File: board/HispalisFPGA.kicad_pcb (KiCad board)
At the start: 4 copper layers, 91.3 x 79.9 mm, 129 parts, among them J1 HC-TYPE-C-16P-01A, Q1 DMG1012T, Q2 DMG1012T, Q3 DMG1012T, Q4 DMG1012T, SW1 SW_DIP_x08, U1 93LC46B, U2 FT2232HQ, Y1 12MHz

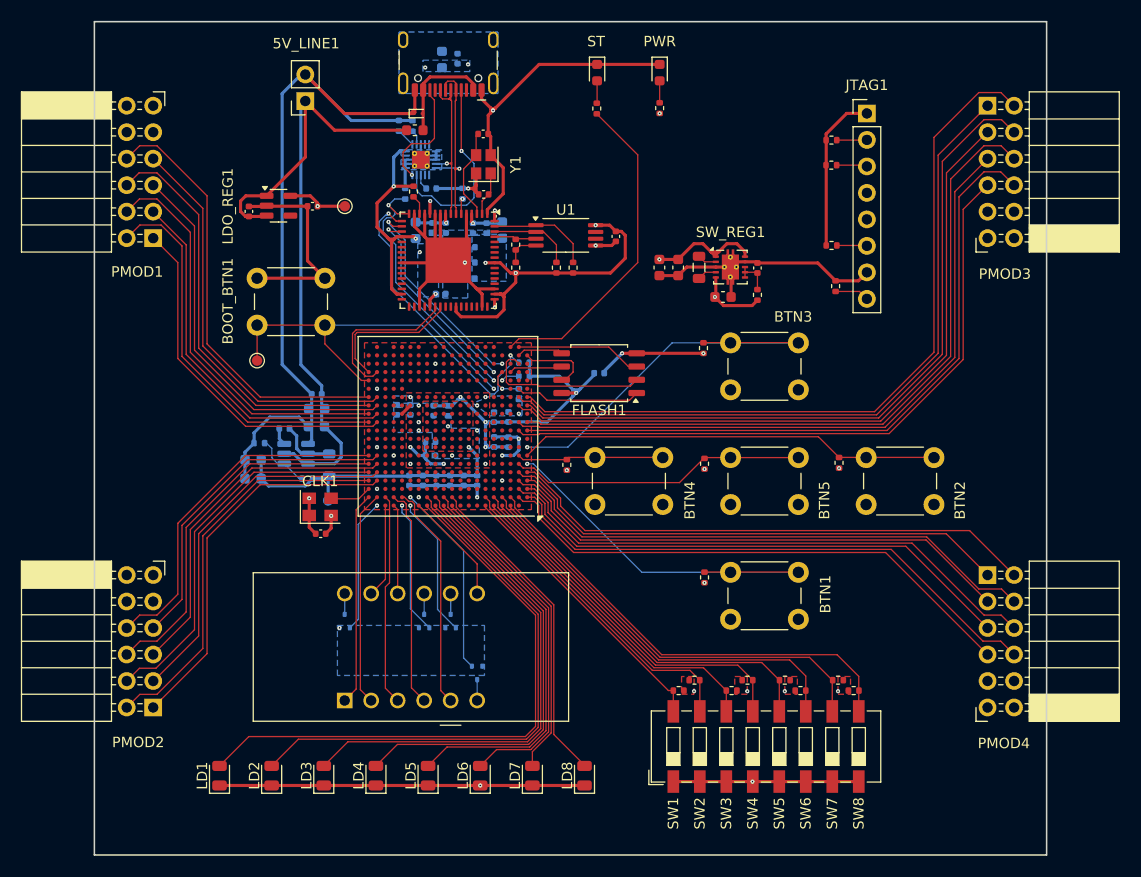
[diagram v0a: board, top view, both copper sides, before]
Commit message: No warnings
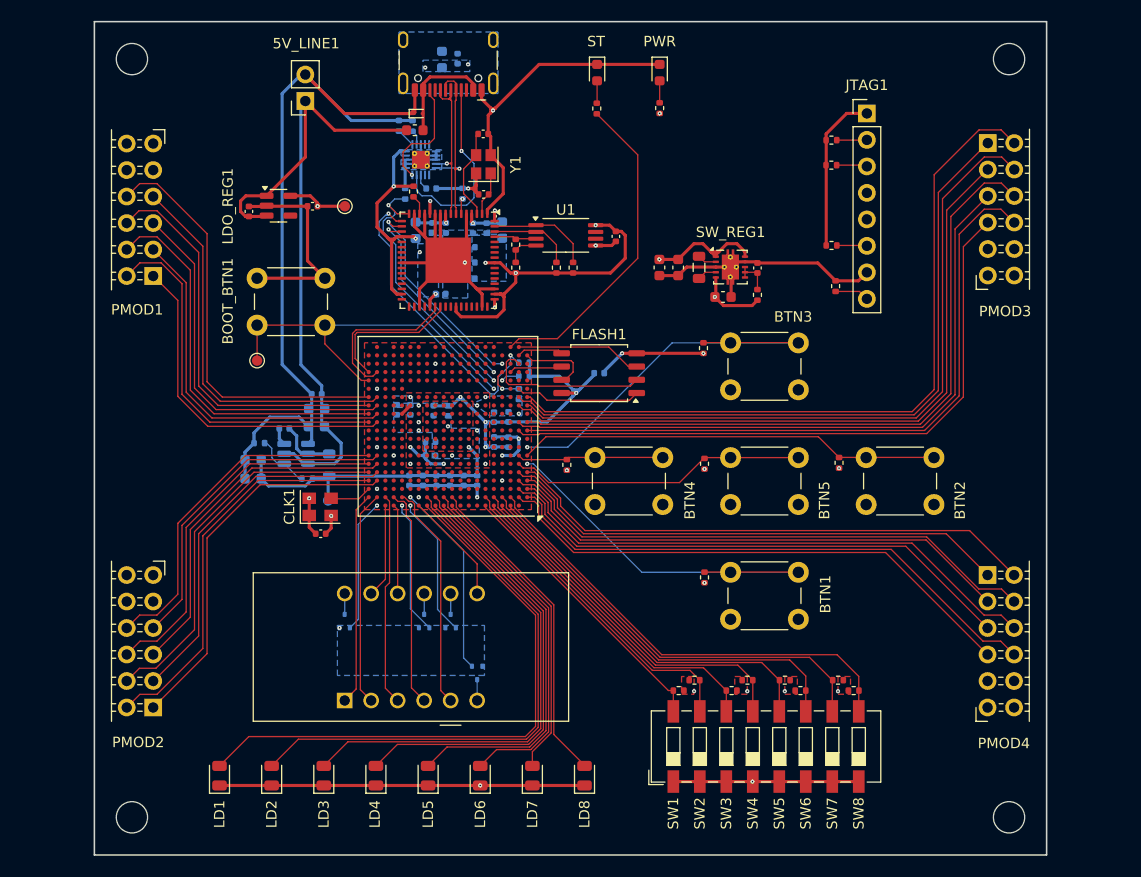
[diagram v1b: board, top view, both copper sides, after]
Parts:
- added MH01: MountingHole_3mm, MountingHole:MountingHole_3mm, F.Cu at (65.9, 107.0)
- added MH02: MountingHole_3mm, MountingHole:MountingHole_3mm, F.Cu at (150.0, 107.0)
- added MH03: MountingHole_3mm, MountingHole:MountingHole_3mm, F.Cu at (65.9, 179.7)
- added MH04: MountingHole_3mm, MountingHole:MountingHole_3mm, F.Cu at (150.0, 179.7)
- moved PMOD1 3.63 mm to (67.9, 115.1)
- moved PMOD3 3.58 mm to (148.0, 127.8)
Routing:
- net PMOD1_9: track 40.4 -> 38.9 mm
- net PMOD1_7: track 37.8 -> 36.3 mm
- net PMOD1_8: track 39.0 -> 37.5 mm
- net PMOD1_4: track 39.0 -> 37.5 mm
- net PMOD1_3: track 37.5 -> 36.0 mm
- net PMOD1_2: track 36.0 -> 34.5 mm
- net PMOD1_1: track 34.5 -> 33.0 mm
- net PMOD1_10: track 42.0 -> 40.5 mm
- net PMOD3_8: track 70.4 -> 68.9 mm
- net PMOD3_7: track 72.5 -> 71.1 mm
- net PMOD3_9: track 68.3 -> 66.8 mm
- net PMOD3_4: track 63.4 -> 62.0 mm
- net PMOD3_3: track 65.1 -> 63.7 mm
- net PMOD3_10: track 66.6 -> 65.1 mm
- net PMOD3_1: track 69.1 -> 67.6 mm
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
